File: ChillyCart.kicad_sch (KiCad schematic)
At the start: 72 parts, among them J1 GameBoy_GamePak_DMG-09, J2 USB_C_Receptacle_USB2.0_16P, J3 Micro_SD_Card_Det1, J4 Conn_01x02_Socket, J5 Conn_01x02_Socket, J7 Conn_01x07_Socket, SW1 SW_Push, U1 TXB0108PW, U10 MCP7940N-x/ST, U11 LSM6DS3, U2 TXB0108PW, U3 TXB0108PW, U4 RP2350_80QFN, U5 AMS1117-3.3, U6 W25Q128JVS, U7 DNF, U8 TPS2111A, U9 TXB0108PW, Y1 ABM8-272-T3, Y2 FC-135

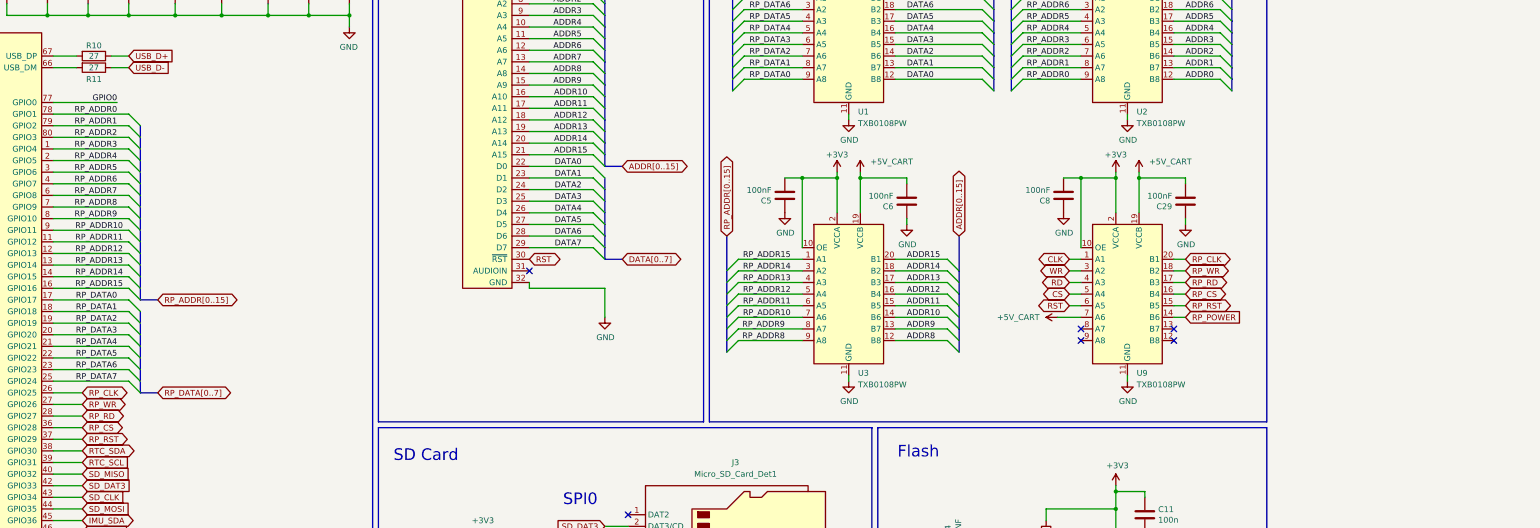
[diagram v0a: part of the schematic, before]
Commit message: Initial routing
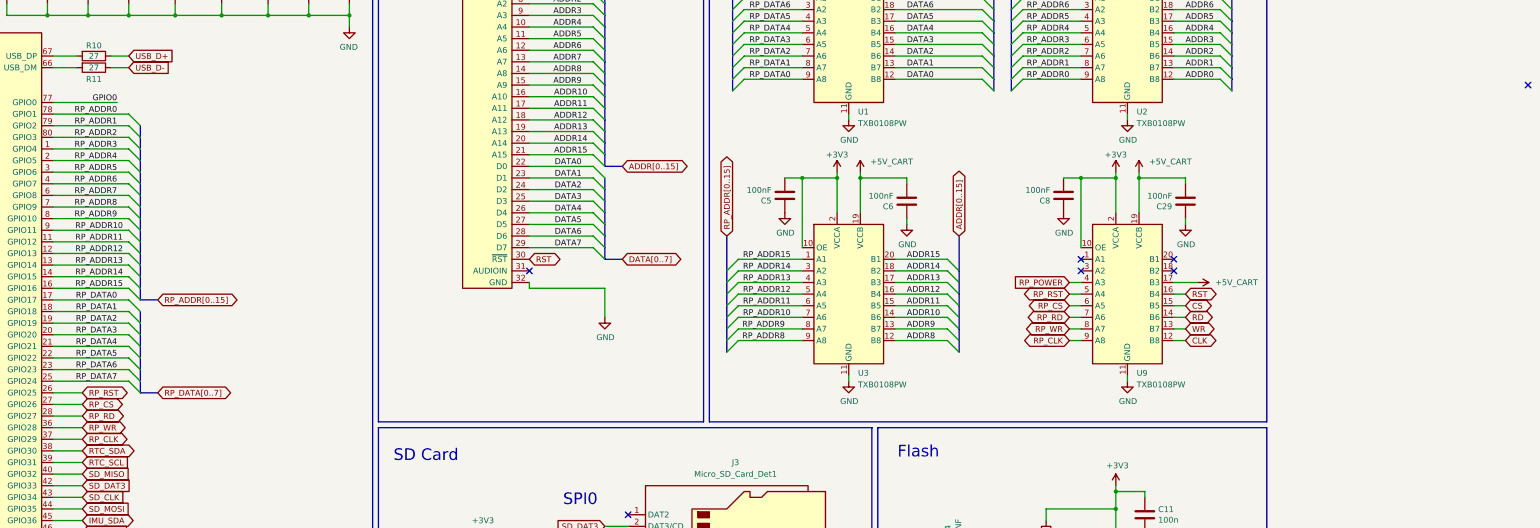
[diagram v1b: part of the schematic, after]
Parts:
- C1, C2, C29, C3, C4, C5, C6, C8: footprint Capacitor_SMD:C_0603_1608Metric_Pad1.08x0.95mm_HandSolder -> Capacitor_SMD:C_0402_1005Metric_Pad0.74x0.62mm_HandSolder
- C10, C11, C12, C13, C14, C15, C16, C17, C18, C19, C20, C21, C24, C25, C26, C27, C9: footprint Capacitor_SMD:C_0402_1005Metric -> Capacitor_SMD:C_0402_1005Metric_Pad0.74x0.62mm_HandSolder
- C22, C23: footprint RP2350_80QFN_minimal:C_0402_1005Metric_small_pads -> Capacitor_SMD:C_0402_1005Metric_Pad0.74x0.62mm_HandSolder
- C28, C34, C35, C36, C7: footprint Capacitor_SMD:C_0805_2012Metric -> Capacitor_SMD:C_0402_1005Metric_Pad0.74x0.62mm_HandSolder
- C30, C31, C32, C33: footprint Capacitor_SMD:C_0603_1608Metric -> Capacitor_SMD:C_0402_1005Metric_Pad0.74x0.62mm_HandSolder
- R1, R10, R11, R14, R15, R2, R3, R4, R5, R6, R7, R8, R9: footprint Resistor_SMD:R_0402_1005Metric -> Resistor_SMD:R_0402_1005Metric_Pad0.72x0.64mm_HandSolder
- R12: footprint Resistor_SMD:R_0603_1608Metric -> Resistor_SMD:R_0402_1005Metric_Pad0.72x0.64mm_HandSolder
- R13: footprint (none) -> Resistor_SMD:R_0402_1005Metric_Pad0.72x0.64mm_HandSolder
- SW1: footprint (none) -> Button_Switch_SMD:SW_Push_1P1T_XKB_TS-1187A
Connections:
- net +5V_CART: now also U9.17 (B3); no longer U9.7 (A6)
- net CLK: now also U9.12 (B8); no longer U9.1 (A1)
- net CS: now also U9.15 (B5); no longer U9.5 (A4)
- net RD: now also U9.14 (B6); no longer U9.4 (A3)
- net RP_CLK: now also U4.37 (GPIO29), U9.9 (A8); no longer U4.26 (GPIO25), U9.20 (B1)
- net RP_CS: now also U4.27 (GPIO26), U9.6 (A5); no longer U4.36 (GPIO28), U9.16 (B4)
- net RP_POWER: now also U9.4 (A3); no longer U9.14 (B6)
- net RP_RD: now also U9.7 (A6); no longer U9.17 (B3)
- net RP_RST: now also U4.26 (GPIO25), U9.5 (A4); no longer U4.37 (GPIO29), U9.15 (B5)
- net RP_WR: now also U4.36 (GPIO28), U9.8 (A7); no longer U4.27 (GPIO26), U9.18 (B2)
- net RST: now also U9.16 (B4); no longer U9.6 (A5)
- net WR: now also U9.13 (B7); no longer U9.3 (A2)
- no-connect marks 14 -> 15
